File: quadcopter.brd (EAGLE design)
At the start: 196 x 196 mm, 65 parts, among them J1 ISP, U2 ATMEGA128RFA1

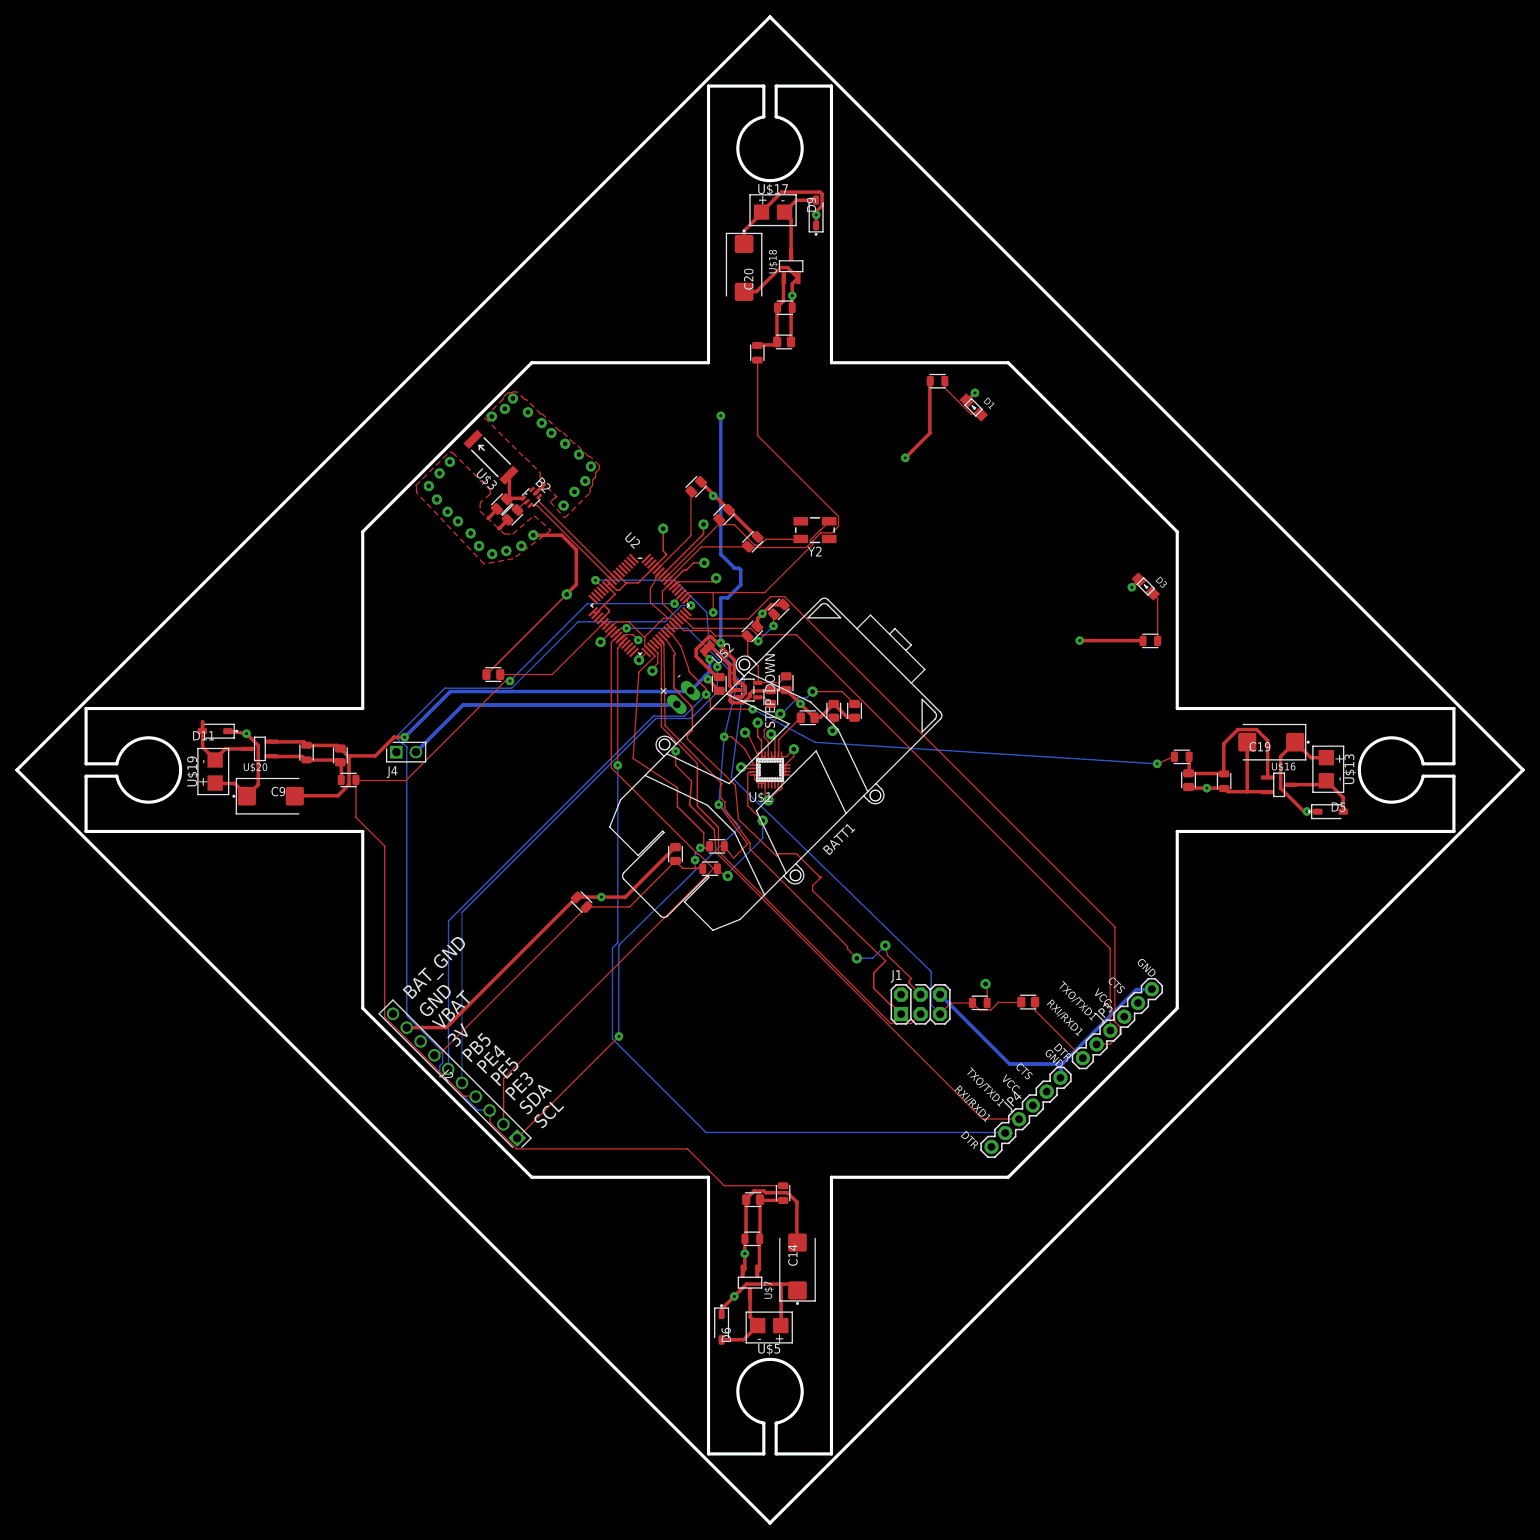
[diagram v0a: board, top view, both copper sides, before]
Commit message: autorouting works, things are good
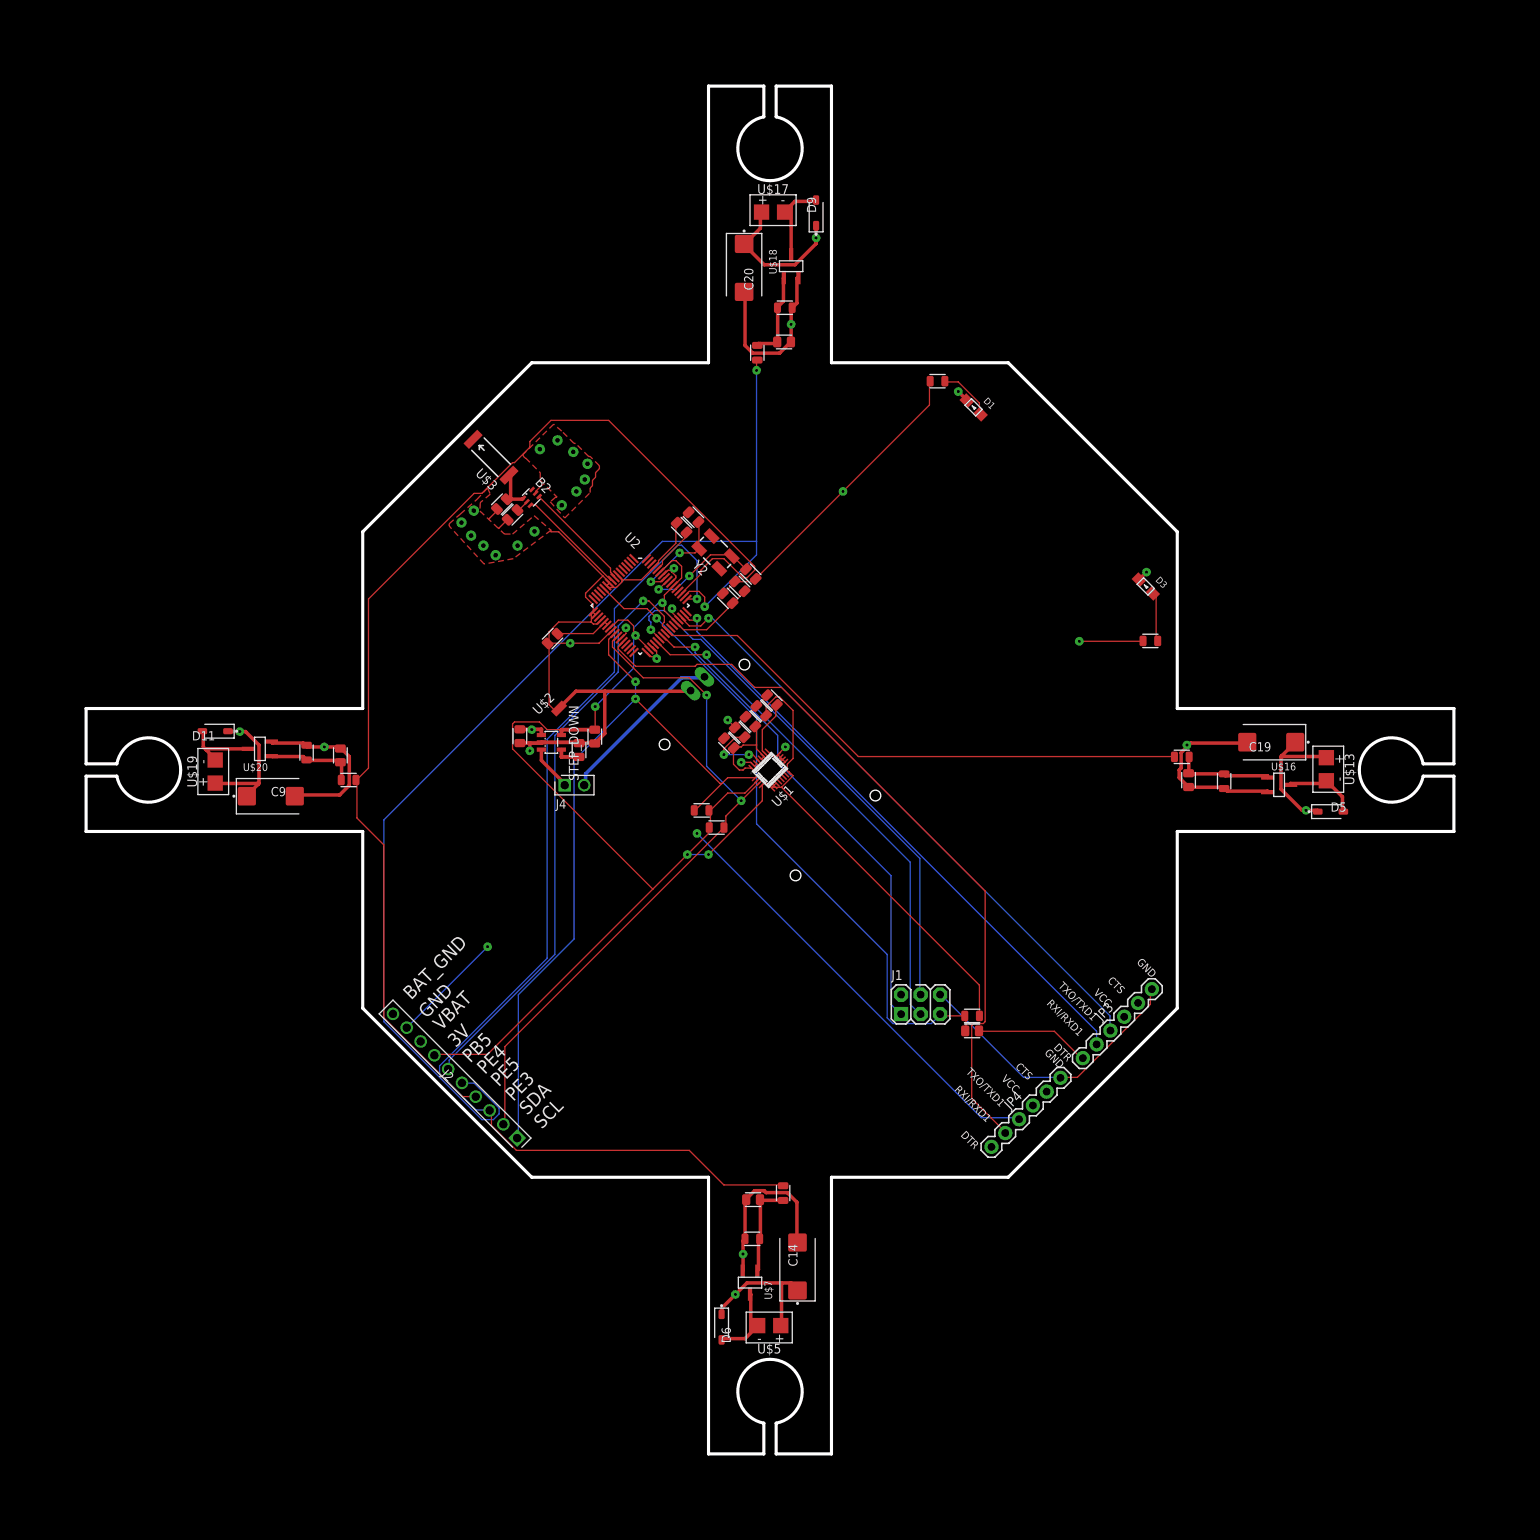
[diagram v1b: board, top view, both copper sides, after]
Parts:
- moved C27 26.8 mm to (-32.5, 4.40)
- moved STEP_DOWN 26.4 mm to (-28.4, 3.60)
- moved C13 25.9 mm to (-24.9, 2.60)
- moved J4 22.3 mm to (-26.7, -1.97)
- moved C28 21.6 mm to (-22.8, 4.35), turned to 270 degrees
- moved U$2 20.8 mm to (-27.4, 8.00), turned to 45 degrees
- moved C11 16.0 mm to (-5.35, 3.50), turned to 135 degrees
- moved C18 15.2 mm to (-3.95, 4.90), turned to 315 degrees
- moved Y2 13.3 mm to (-7.09, 28.3), turned to 135 degrees
- moved C16 10.9 mm to (-2.55, 6.30), turned to 135 degrees
- moved C5 9.01 mm to (-28.3, 17.1), turned to 225 degrees
- moved C12 8.21 mm to (26.3, -34.0)
- moved C3 5.92 mm to (-3.95, 23.9), turned to 135 degrees
- moved C6 5.63 mm to (-11.5, 31.6), turned to 135 degrees
- moved R7 5.42 mm to (-6.95, -7.49)
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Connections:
- net BAT_GND: now also C13.2, C28.2, STEP_DOWN.2
- net GND: no longer C13.2, C28.2, STEP_DOWN.2
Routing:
- net 3V: track 157.3 -> 244.3 mm, vias 11 -> 5
- net PE5: track 101.2 -> 154.8 mm, vias 2 -> 0
- net GND: track 241.5 -> 197.2 mm, vias 39 -> 24
- net VBAT: track 125.6 -> 87.4 mm, vias 8 -> 7
- net PE4: track 130.6 -> 156.7 mm
- net JUMPER_INPUT: track 36.5 -> 22.2 mm
- net TXD1: track 93.1 -> 79.1 mm, vias 0 -> 1
- net TX1: track 108.5 -> 97.0 mm, vias 1 -> 0
- net PB5: track 138.9 -> 150.1 mm, vias 3 -> 1
- net FILTERED: track 22.6 -> 12.8 mm
- net RESET: track 95.7 -> 86.1 mm
- net DVDD: track 16.9 -> 7.31 mm
- net N$3: track 23.2 -> 13.7 mm, vias 0 -> 2
- net SCL: track 109.0 -> 99.4 mm, vias 4 -> 2
- net SDA: track 100.1 -> 90.6 mm
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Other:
- board size 196 x 196 mm -> 178 x 178 mm

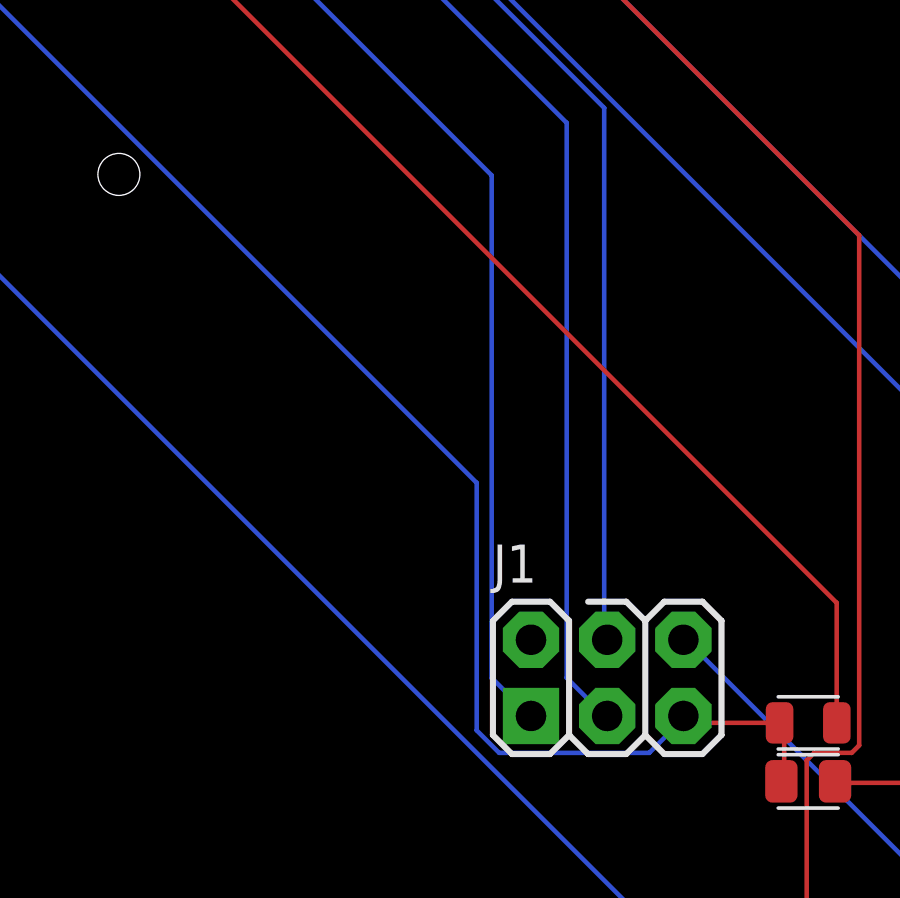
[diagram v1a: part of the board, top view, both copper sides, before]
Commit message: almost forgot newest board and schematic
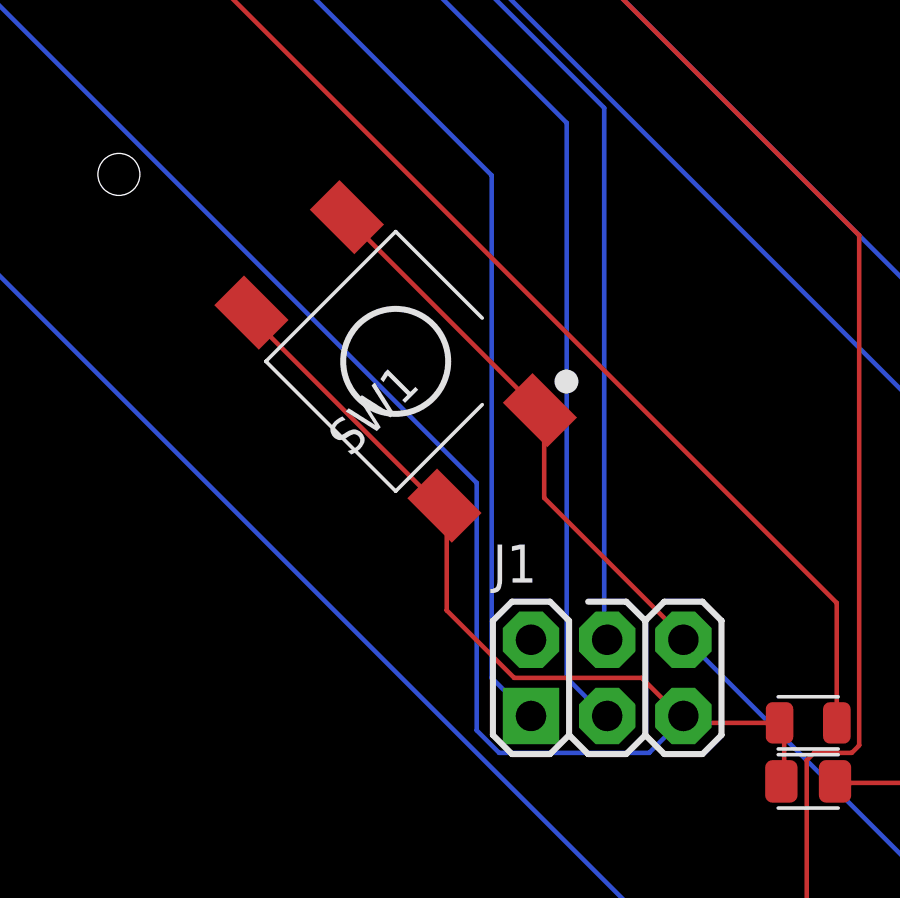
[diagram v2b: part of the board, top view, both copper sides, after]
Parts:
- added SW1: PUSHBUTTON_SMD-VERTICAL-1, quadparts_prebuilt:TE_FSM8JSMA_HS
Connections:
- net GND: now also SW1.1, SW1.2
- net RESET: now also SW1.3, SW1.4
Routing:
- net RESET: track 86.1 -> 108.1 mm
- net GND: track 197.2 -> 216.0 mm
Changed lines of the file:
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@@
 <attribute name="PRICE" value="10.21" x="-16.9" y="21.4" size="1.778" layer="27" rot="R315" display="off"/>
+</element>
+<element name="SW1" library="quadparts_prebuilt" package="TE_FSM8JSMA_HS" value="PUSHBUTTON_SMD-VERTICAL-1" x="12.55" y="-19.95" rot="R225">
+<attribute name="DIST" value="Digikey" x="12.55" y="-19.95" size="1.778" layer="27" rot="R225" display="off"/>
+<attribute name="DISTPN" value="450-1129-ND" x="12.55" y="-19.95" size="1.778" layer="27" rot="R225" display="off"/>
+<attribute name="MFR" value="TE Connectivity Alcoswitch Switches" x="12.55" y="-19.95" size="1.778" layer="27" rot="R225" display="off"/>
+<attribute name="MPN" value="FSM4JSMA" x="12.55" y="-19.95" size="1.778" layer="27" rot="R225" display="off"/>
 </element>
 </elements>
@@
 <wire x1="-28" y1="7.75" x2="-27.803553125" y2="7.64644375" width="0.1524" layer="1"/>
 <wire x1="-28.75" y1="16.25" x2="-28.932859375" y2="16.4671375" width="0.1524" layer="1"/>
+<contactref element="SW1" pad="2"/>
+<contactref element="SW1" pad="1"/>
+<wire x1="11" y1="-15.25" x2="17.25" y2="-21.5" width="0.1524" layer="1"/>
+<wire x1="17.25" y1="-21.5" x2="17.358325" y2="-21.57634375" width="0.1524" layer="1"/>
+<wire x1="11" y1="-15.25" x2="10.923653125" y2="-15.141671875" width="0.1524" layer="1"/>
+<wire x1="17.5" y1="-24.5" x2="17.5" y2="-21.75" width="0.1524" layer="1"/>
+<wire x1="22" y1="-29" x2="17.5" y2="-24.5" width="0.1524" layer="1"/>
+<wire x1="17.5" y1="-21.75" x2="17.358325" y2="-21.57634375" width="0.1524" layer="1"/>
+<wire x1="22" y1="-29" x2="22.14" y2="-29.23" width="0.1524" layer="1"/>
 </signal>
 <signal name="N$3">
@@
 <wire x1="22.25" y1="-32" x2="22.14" y2="-31.77" width="0.1524" layer="1"/>
 <via x="-14.75" y="19.75" extent="1-16" drill="0.381"/>
+<contactref element="SW1" pad="4"/>
+<contactref element="SW1" pad="3"/>
+<wire x1="14" y1="-24.75" x2="7.75" y2="-18.5" width="0.1524" layer="1"/>
+<wire x1="7.75" y1="-18.5" x2="7.741671875" y2="-18.323653125" width="0.1524" layer="1"/>
+<wire x1="14" y1="-24.75" x2="14.17634375" y2="-24.758325" width="0.1524" layer="1"/>
+<wire x1="14.25" y1="-28.25" x2="14.25" y2="-25" width="0.1524" layer="1"/>
+<wire x1="16.5" y1="-30.5" x2="14.25" y2="-28.25" width="0.1524" layer="1"/>
+<wire x1="20.75" y1="-30.5" x2="16.5" y2="-30.5" width="0.1524" layer="1"/>
+<wire x1="22" y1="-31.75" x2="20.75" y2="-30.5" width="0.1524" layer="1"/>
+<wire x1="14.25" y1="-25" x2="14.17634375" y2="-24.758325" width="0.1524" layer="1"/>
+<wire x1="22" y1="-31.75" x2="22.14" y2="-31.77" width="0.1524" layer="1"/>
 </signal>
 <signal name="PE5">
